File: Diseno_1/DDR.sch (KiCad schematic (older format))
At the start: 23 parts, among them U5 XC7Z010-BUENO, U6 MT41K256M16TW-107_P

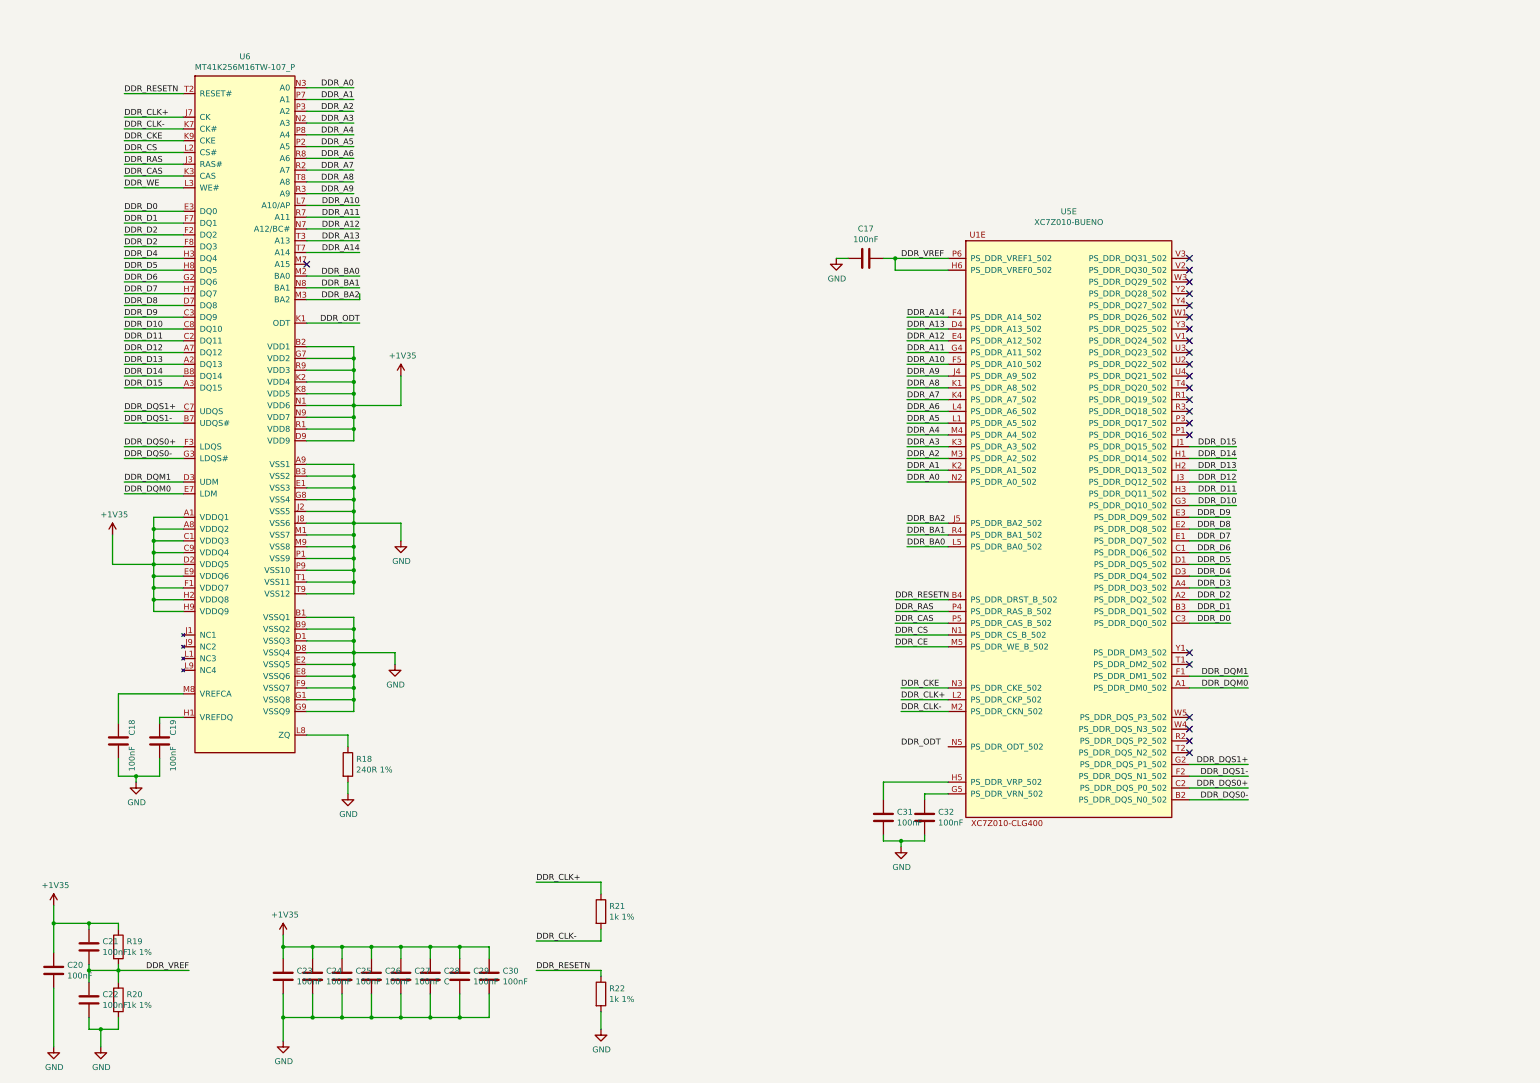
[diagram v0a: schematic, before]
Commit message: actualizacion
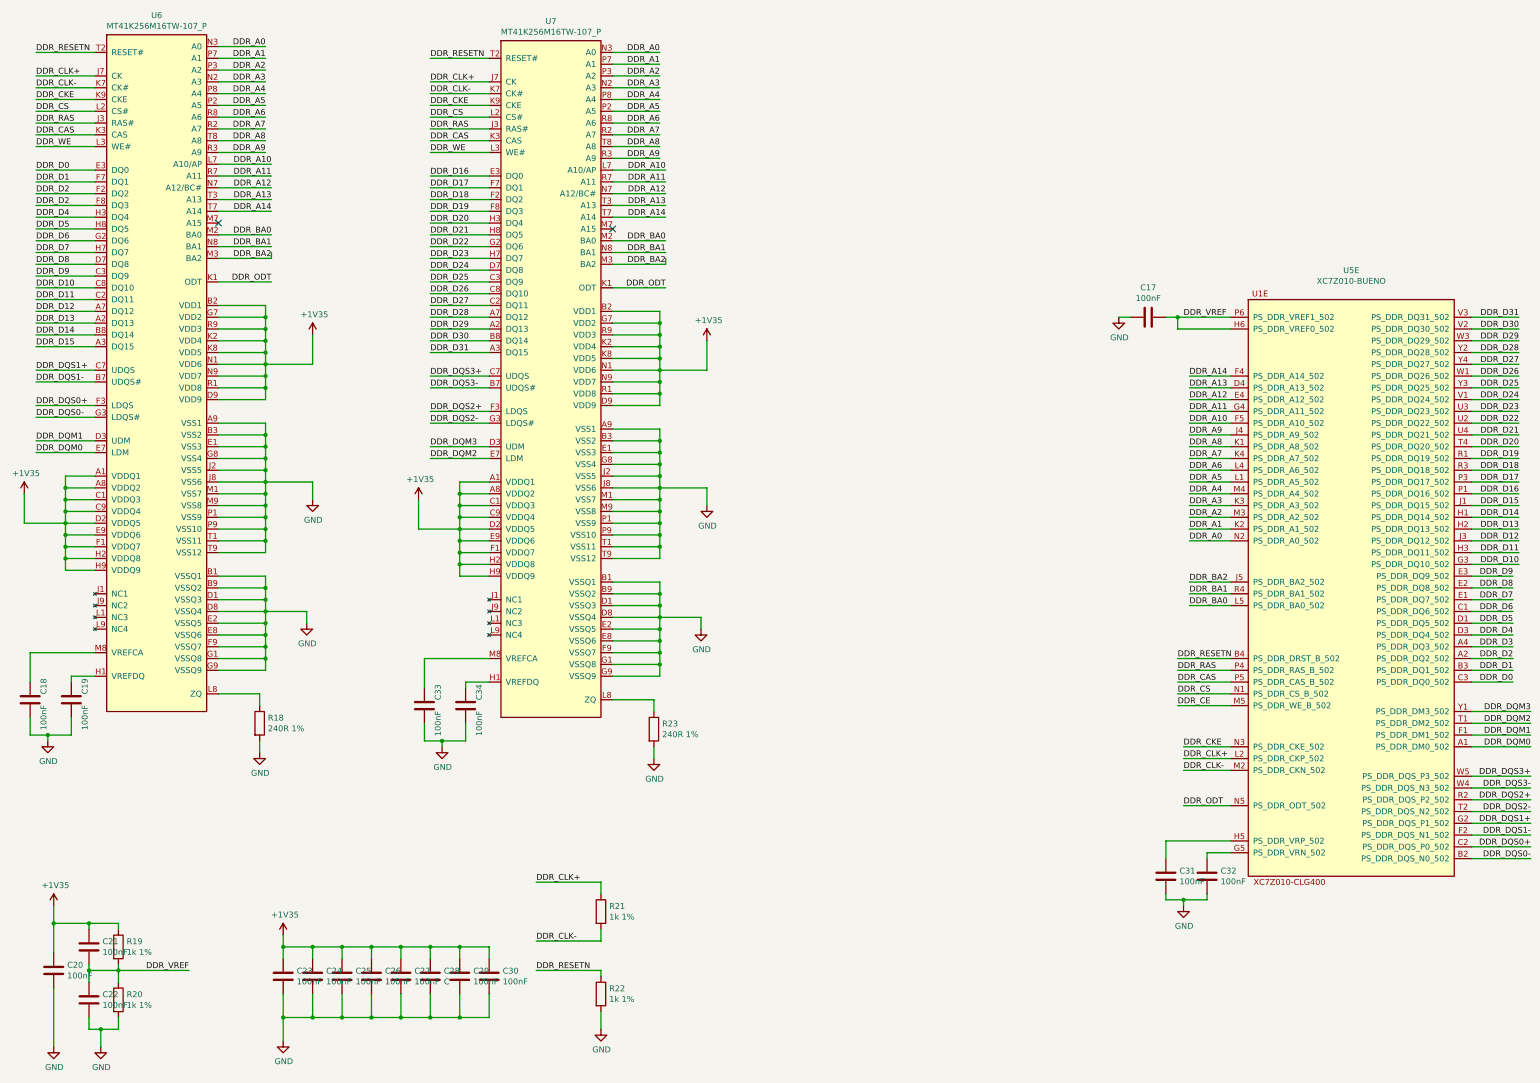
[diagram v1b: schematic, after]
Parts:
- added C33, C34: 100nF, Capacitor_SMD:C_0805_2012Metric, symbol Device:C
- added R23: 240R 1%, Resistor_SMD:R_0805_2012Metric, symbol Device:R
- added U7: MT41K256M16TW-107_P, ZYNQ_7000:BGA-144_9x16_8.0x14.0mm, symbol Zynq_7000:MT41K256M16TW-107_P
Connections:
- net +1V35: now also U7.A1 (VDDQ1), U7.A8 (VDDQ2), U7.B2 (VDD1), U7.C1 (VDDQ3), U7.C9 (VDDQ4), U7.D2 (VDDQ5), U7.D9 (VDD9), U7.E9 (VDDQ6), U7.F1 (VDDQ7), U7.G7 (VDD2), U7.H2 (VDDQ8), U7.H9 (VDDQ9), U7.K2 (VDD4), U7.K8 (VDD5), U7.N1 (VDD6), U7.N9 (VDD7), U7.R1 (VDD8), U7.R9 (VDD3)
- net DDR_A0: now also U7.N3 (A0)
- net DDR_A1: now also U7.P7 (A1)
- net DDR_A10: now also U7.L7 (A10/AP)
- net DDR_A11: now also U7.R7 (A11)
- net DDR_A12: now also U7.N7 (A12/BC#)
- net DDR_A13: now also U7.T3 (A13)
- net DDR_A14: now also U7.T7 (A14)
- net DDR_A2: now also U7.P3 (A2)
- net DDR_A3: now also U7.N2 (A3)
- net DDR_A4: now also U7.P8 (A4)
- net DDR_A5: now also U7.P2 (A5)
- net DDR_A6: now also U7.R8 (A6)
- net DDR_A7: now also U7.R2 (A7)
- net DDR_A8: now also U7.T8 (A8)
- net DDR_A9: now also U7.R3 (A9)
- net DDR_BA0: now also U7.M2 (BA0)
- net DDR_BA1: now also U7.N8 (BA1)
- net DDR_BA2: now also U7.M3 (BA2)
- net DDR_CAS: now also U7.K3 (CAS)
- net DDR_CKE: now also U7.K9 (CKE)
- net DDR_CLK+: now also U7.J7 (CK)
- net DDR_CLK-: now also U7.K7 (CK#)
- net DDR_CS: now also U7.L2 (CS#)
- net DDR_ODT: now also U5.N5 (PS_DDR_ODT_502), U7.K1 (ODT)
- net DDR_RAS: now also U7.J3 (RAS#)
- net DDR_RESETN: now also U7.T2 (RESET#)
- net DDR_WE: now also U7.L3 (WE#)
- net GND: now also C33.2, C34.2, R23.2, U7.A9 (VSS1), U7.B1 (VSSQ1), U7.B3 (VSS2), U7.B9 (VSSQ2), U7.D1 (VSSQ3), U7.D8 (VSSQ4), U7.E1 (VSS3), U7.E2 (VSSQ5), U7.E8 (VSSQ6), U7.F9 (VSSQ7), U7.G1 (VSSQ8), U7.G8 (VSS4), U7.G9 (VSSQ9), U7.J2 (VSS5), U7.J8 (VSS6), U7.M1 (VSS7), U7.M9 (VSS8), U7.P1 (VSS9), U7.P9 (VSS10), U7.T1 (VSS11), U7.T9 (VSS12)
- net DDR_D16: now reaches U5.P1 (PS_DDR_DQ16_502)
- net DDR_D16: now also U7.E3 (DQ0)
- net DDR_D17: now reaches U5.P3 (PS_DDR_DQ17_502)
- net DDR_D17: now also U7.F7 (DQ1)
- net DDR_D19: now reaches U5.R1 (PS_DDR_DQ19_502)
- net DDR_D19: now also U7.F8 (DQ3)
- net DDR_DQS2+: now reaches U5.R2 (PS_DDR_DQS_P2_502)
- net DDR_DQS2+: now also U7.F3 (LDQS)
- net DDR_D18: now reaches U5.R3 (PS_DDR_DQ18_502)
- net DDR_D18: now also U7.F2 (DQ2)
- net DDR_DQM2: now reaches U5.T1 (PS_DDR_DM2_502)
- net DDR_DQM2: now also U7.E7 (LDM)
- net DDR_DQS2-: now reaches U5.T2 (PS_DDR_DQS_N2_502)
- net DDR_DQS2-: now also U7.G3 (LDQS#)
- net DDR_D20: now reaches U5.T4 (PS_DDR_DQ20_502)
- net DDR_D20: now also U7.H3 (DQ4)
- net DDR_D22: now reaches U5.U2 (PS_DDR_DQ22_502)
- net DDR_D22: now also U7.G2 (DQ6)
- net DDR_D23: now reaches U5.U3 (PS_DDR_DQ23_502)
- net DDR_D23: now also U7.H7 (DQ7)
- net DDR_D21: now reaches U5.U4 (PS_DDR_DQ21_502)
- net DDR_D21: now also U7.H8 (DQ5)
- net DDR_D24: now reaches U5.V1 (PS_DDR_DQ24_502)
- net DDR_D24: now also U7.D7 (DQ8)
- net DDR_D30: now reaches U5.V2 (PS_DDR_DQ30_502)
- net DDR_D30: now also U7.B8 (DQ14)
- net DDR_D31: now reaches U5.V3 (PS_DDR_DQ31_502)
- net DDR_D31: now also U7.A3 (DQ15)
- net DDR_D26: now reaches U5.W1 (PS_DDR_DQ26_502)
- net DDR_D26: now also U7.C8 (DQ10)
- net DDR_D29: now reaches U5.W3 (PS_DDR_DQ29_502)
- net DDR_D29: now also U7.A2 (DQ13)
- net DDR_DQS3-: now reaches U5.W4 (PS_DDR_DQS_N3_502)
- net DDR_DQS3-: now also U7.B7 (UDQS#)
- net DDR_DQS3+: now reaches U5.W5 (PS_DDR_DQS_P3_502)
- net DDR_DQS3+: now also U7.C7 (UDQS)
- net DDR_DQM3: now reaches U5.Y1 (PS_DDR_DM3_502)
- net DDR_DQM3: now also U7.D3 (UDM)
- net DDR_D28: now reaches U5.Y2 (PS_DDR_DQ28_502)
- net DDR_D28: now also U7.A7 (DQ12)
- net DDR_D25: now reaches U5.Y3 (PS_DDR_DQ25_502)
- net DDR_D25: now also U7.C3 (DQ9)
- net DDR_D27: now reaches U5.Y4 (PS_DDR_DQ27_502)
- net DDR_D27: now also U7.C2 (DQ11)
- new net: C34.1, U7.H1 (VREFDQ)
- new net: R23.1, U7.L8 (ZQ)
- new net: C33.1, U7.M8 (VREFCA)
- no-connect marks 23 -> 2
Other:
- moved on the sheet: C17, C18, C19, C31, C32, R18, U5E, U6
